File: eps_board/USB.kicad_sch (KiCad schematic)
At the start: 3 parts, among them J12 10155435-00011LF

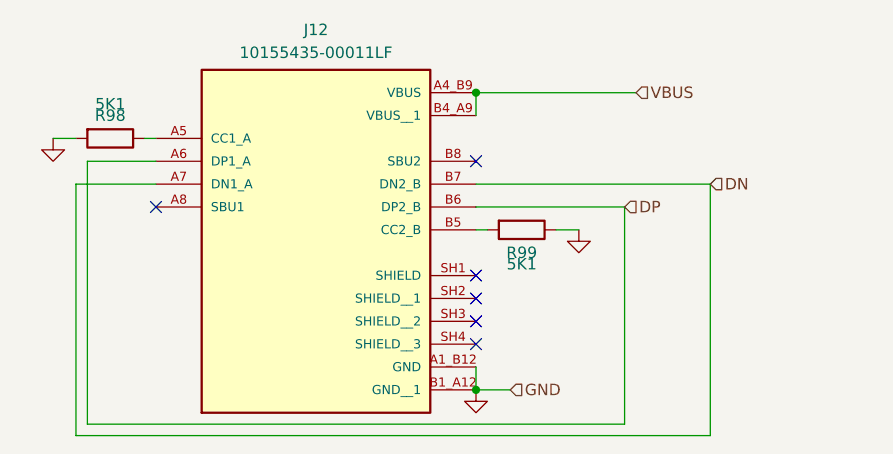
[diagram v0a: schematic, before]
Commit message: laying all the tracks, interim commit
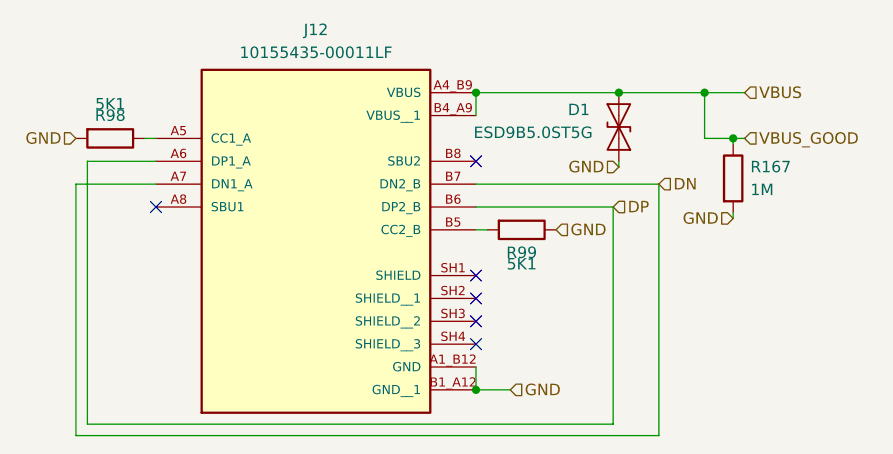
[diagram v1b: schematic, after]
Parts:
- added D1: ESD9B5.0ST5G, Diode_SMD:D_SOD-923, symbol Diode:ESD9B5.0ST5G
- added R167: 1M, Resistor_SMD:R_0402_1005Metric_Pad0.72x0.64mm_HandSolder, symbol Device:R
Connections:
- net GND: now also D1.2 (A2), R167.2
- net VBUS: now also D1.1 (A1), R167.1

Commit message: interim commit
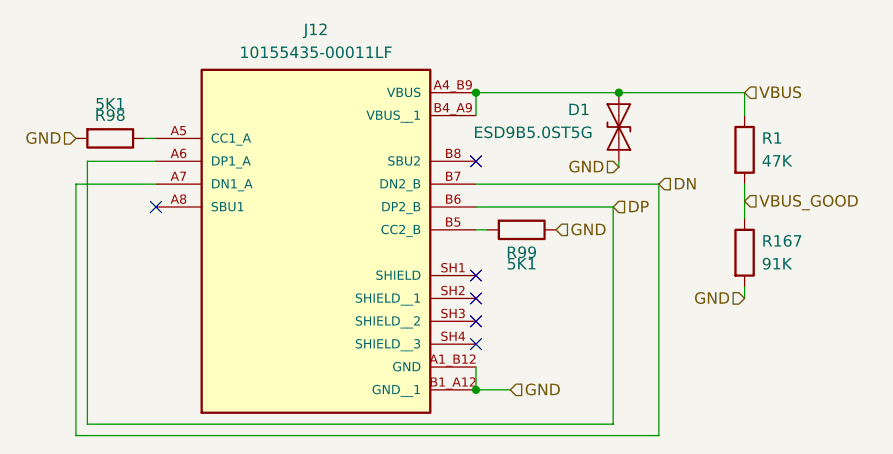
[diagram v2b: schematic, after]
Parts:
- added R1: 47K, Resistor_SMD:R_0402_1005Metric_Pad0.72x0.64mm_HandSolder, symbol Device:R
- R167: value 1M -> 91K
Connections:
- net VBUS: now also R1.1; no longer R167.1
- new net VBUS_GOOD: R1.2, R167.1
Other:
- moved on the sheet: R167
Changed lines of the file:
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@@
 	(paper "A4")
-	(junction
-		(at 189.865 83.185)
-		(diameter 0)
-		(color 0 0 0 0)
-	)
 	(junction
 		(at 177.165 78.105)
@@
 		(color 0 0 0 0)
 	)
-	(junction
-		(at 186.69 78.105)
-		(diameter 0)
-		(color 0 0 0 0)
-	)
 	(no_connect
 		(at 161.29 106.045)
@@
 	(wire
 		(pts
-			(xy 189.865 83.82) (xy 189.865 83.185)
-		)
-		(stroke
-			(width 0)
-			(type default)
-		)
-	)
-	(wire
-		(pts
-			(xy 189.865 83.185) (xy 191.135 83.185)
-		)
-		(stroke
-			(width 0)
-			(type default)
-		)
-	)
-	(wire
-		(pts
-			(xy 177.165 78.105) (xy 186.69 78.105)
+			(xy 177.165 78.105) (xy 191.135 78.105)
 		)
 		(stroke
@@
 	(wire
 		(pts
-			(xy 189.865 92.075) (xy 189.865 91.44)
-		)
-		(stroke
-			(width 0)
-			(type default)
-		)
-	)
-	(wire
-		(pts
-			(xy 186.69 83.185) (xy 189.865 83.185)
+			(xy 191.135 100.965) (xy 191.135 99.695)
 		)
 		(stroke
@@
 	(wire
 		(pts
+			(xy 191.135 88.265) (xy 191.135 92.075)
+		)
+		(stroke
+			(width 0)
+			(type default)
+		)
+	)
+	(wire
+		(pts
 			(xy 177.165 86.36) (xy 177.165 85.725)
 		)
@@
 	(wire
 		(pts
-			(xy 186.69 78.105) (xy 186.69 83.185)
-		)
-		(stroke
-			(width 0)
-			(type default)
-		)
-	)
-	(wire
-		(pts
-			(xy 186.69 78.105) (xy 191.135 78.105)
+			(xy 191.135 78.105) (xy 191.135 80.645)
 		)
 		(stroke
@@
 		)
 	)
+	(hierarchical_label "VBUS_GOOD"
+		(shape input)
+		(at 191.135 90.17 0)
+		(fields_autoplaced yes)
+		(effects
+			(font
+				(size 1.27 1.27)
+			)
+			(justify left)
+		)
+	)
 	(hierarchical_label "VBUS"
 		(shape input)
@@
 		)
 	)
-	(hierarchical_label "VBUS_GOOD"
+	(hierarchical_label "GND"
 		(shape input)
-		(at 191.135 83.185 0)
+		(at 191.135 100.965 180)
 		(fields_autoplaced yes)
 		(effects
@@
 				(size 1.27 1.27)
 			)
-			(justify left)
-		)
-	)
-	(hierarchical_label "GND"
+			(justify right)
+		)
+	)
+	(hierarchical_label "DN"
 		(shape input)
-		(at 189.865 92.075 180)
+		(at 181.61 88.265 0)
 		(fields_autoplaced yes)
 		(effects
@@
 				(size 1.27 1.27)
 			)
-			(justify right)
-		)
-	)
-	(hierarchical_label "DN"
-		(shape input)
-		(at 181.61 88.265 0)
-		(fields_autoplaced yes)
-		(effects
-			(font
-				(size 1.27 1.27)
-			)
 			(justify left)
+		)
+	)
+	(symbol
+		(lib_id "Device:R")
+		(at 191.135 84.455 0)
+		(unit 1)
+		(exclude_from_sim no)
+		(in_bom yes)
+		(on_board yes)
+		(dnp no)
+		(fields_autoplaced yes)
+		(property "Reference" "R1"
+			(at 193.04 83.1849 0)
+			(effects
+				(font
+					(size 1.27 1.27)
+				)
+				(justify left)
+			)
+		)
+		(property "Value" "47K"
+			(at 193.04 85.7249 0)
+			(effects
+				(font
+					(size 1.27 1.27)
+				)
+				(justify left)
+			)
+		)
+		(property "Footprint" "Resistor_SMD:R_0402_1005Metric_Pad0.72x0.64mm_HandSolder"
+			(at 189.357 84.455 90)
+			(effects
+				(font
+					(size 1.27 1.27)
+				)
+				(hide yes)
+			)
+		)
+		(property "Datasheet" "~"
+			(at 191.135 84.455 0)
+			(effects
+				(font
+					(size 1.27 1.27)
+				)
+				(hide yes)
+			)
+		)
+		(property "Description" "Resistor"
+			(at 191.135 84.455 0)
+			(effects
+				(font
+					(size 1.27 1.27)
+				)
+				(hide yes)
+			)
+		)
+		(pin "1"
+		)
+		(pin "2"
+		)
+		(instances
+			(project "EPS"
+				(path "/05170af6-30ef-4c3a-b972-f098085da1bc/dffa178b-07a8-4735-b10c-32a6042c7f6e"
+					(reference "R1")
+					(unit 1)
+				)
+			)
 		)
 	)
@@
 	(symbol
 		(lib_id "Device:R")
-		(at 189.865 87.63 0)
+		(at 191.135 95.885 0)
 		(unit 1)
 		(exclude_from_sim no)
@@
 		(fields_autoplaced yes)
 		(property "Reference" "R167"
-			(at 191.77 86.3599 0)
+			(at 193.04 94.6149 0)
 			(effects
 				(font
@@
 			)
 		)
-		(property "Value" "1M"
-			(at 191.77 88.8999 0)
+		(property "Value" "91K"
+			(at 193.04 97.1549 0)
 			(effects
 				(font
@@
 		)
 		(property "Footprint" "Resistor_SMD:R_0402_1005Metric_Pad0.72x0.64mm_HandSolder"
-			(at 188.087 87.63 90)
+			(at 189.357 95.885 90)
 			(effects
 				(font
@@
 		)
 		(property "Datasheet" "~"
-			(at 189.865 87.63 0)
+			(at 191.135 95.885 0)
 			(effects
 				(font
@@
 		)
 		(property "Description" "Resistor"
-			(at 189.865 87.63 0)
-			(effects
-				(font
+			(at 191.135 95.885 0)
+			(effects
+				(font
